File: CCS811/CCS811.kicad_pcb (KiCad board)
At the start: 2 copper layers, 18 x 20.1 mm, 28 parts, among them J1 Conn_01x04, J2 Conn_01x04, Q1 BSS138DW, Q2 BSS138, Q3 BSS138DW, U1 AP2127K-3.3, U2 CCS811

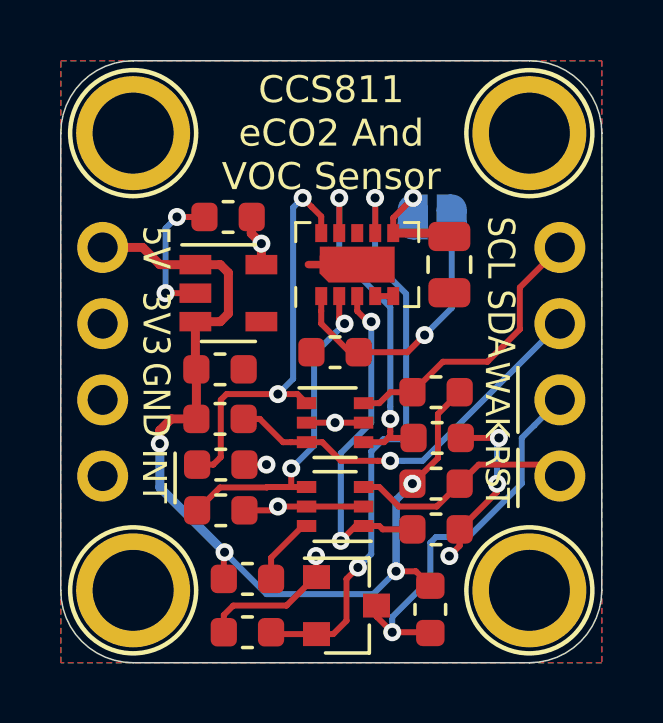
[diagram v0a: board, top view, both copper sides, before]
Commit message: Minor Layout Updates
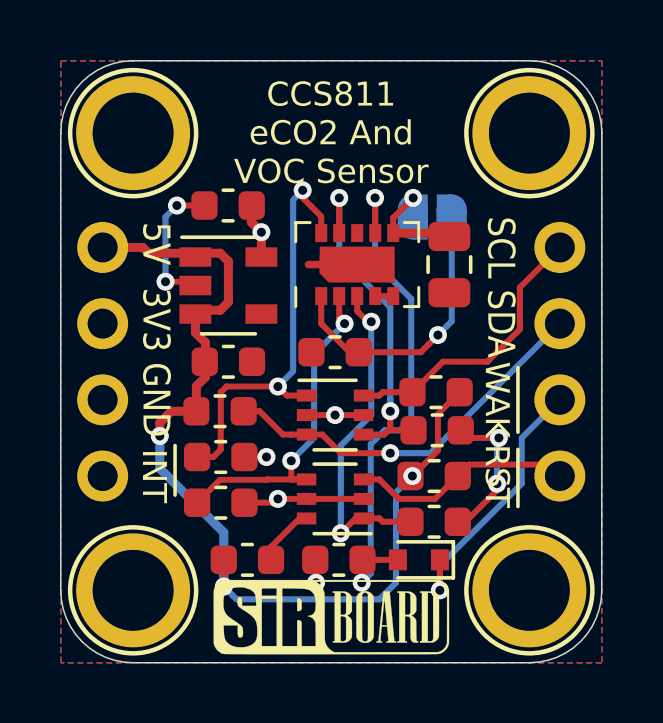
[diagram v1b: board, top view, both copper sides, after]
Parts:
- removed Q3: BSS138DW, Package_TO_SOT_SMD:SOT-363_SC-70-6
- removed R10: 4K7, Resistor_SMD:R_0603_1608Metric
- added D1: 1N4148, Diode_SMD:D_SOD-523, F.Cu at (67.2, 39.8)
- added G***: LOGO, logo:SirBoard79x25, F.Cu at (64.3, 41.7)
- Q2: value BSS138 -> BSS138DW; footprint Package_TO_SOT_SMD:SOT-23 -> Package_TO_SOT_SMD:SOT-363_SC-70-6
- R8: value 4K7 -> 100K
- moved R7 7.23 mm to (60.6, 37.8)
- moved R9 7.20 mm to (67.7, 37.0)
- moved Q2 3.58 mm to (64.4, 37.7), turned to 180 degrees
- moved R8 3.11 mm to (64.5, 39.8)
- moved R5 2.92 mm to (67.7, 38.5), turned to 0 degrees
- moved R6 2.41 mm to (61.5, 39.8), turned to 0 degrees
- moved C3 0.38 mm to (60.8, 27.9)
- moved C1 0.38 mm to (60.8, 33.1)
- moved Q1 0.25 mm to (64.4, 34.9)
- moved U1 0.25 mm to (60.8, 30.6)
- moved R1 0.25 mm to (60.6, 36.3)
- moved R3 0.25 mm to (67.8, 35.4)
- moved R4 0.25 mm to (60.6, 34.8)
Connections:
- Q2 pad 1: 3V3 -> nINT3V3
- Q2 pad 2: nWake_3V3 -> 3V3
- Q2 pad 3: nWake_5V -> nRST_5V
- R5 pad 1: 5V -> nINT3V3
- R5 pad 2: nWake_5V -> 3V3
- R6 pad 1: nWake_3V3 -> 5V
- R6 pad 2: 3V3 -> nINT_5V
- R7 pad 1: nINT3V3 -> nRST_3V3
- R8 pad 1: 5V -> 3V3
- R8 pad 2: nINT_5V -> nWake_3V3
- R9 pad 1: nRST_3V3 -> 5V
- R9 pad 2: 3V3 -> nRST_5V
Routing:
- net 3V3: track 22.6 -> 17.5 mm, vias 9 -> 8
- net nWake_5V: track 13.1 -> 8.77 mm
- net nWake_3V3: track 19.7 -> 17.4 mm
- net 5V: track 32.4 -> 32.7 mm, vias 4 -> 3
